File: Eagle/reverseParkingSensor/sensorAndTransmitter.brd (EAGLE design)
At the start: 42.2 x 52.1 mm, 31 parts, among them IC1 LM393N, IC3 MEGA8-P, Q1 BC558B, T1 BPX81, X1 YH-55-10

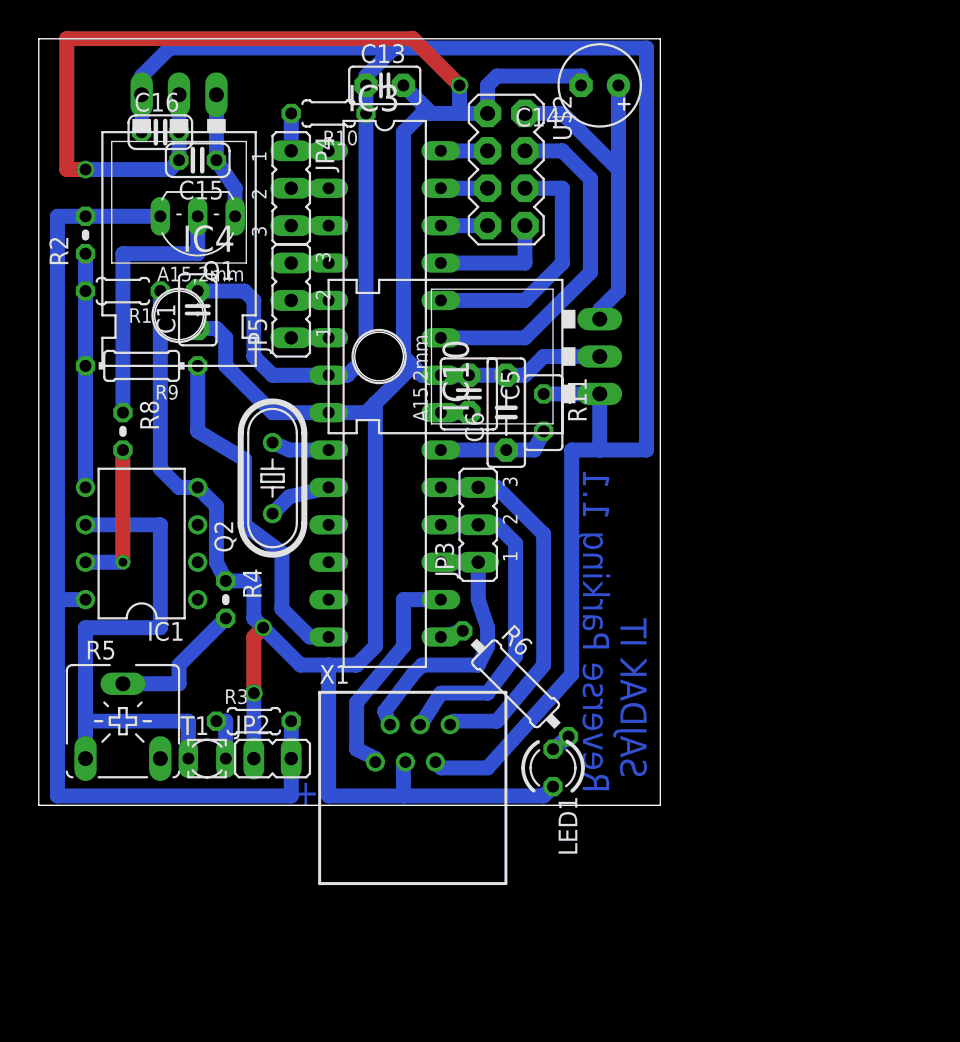
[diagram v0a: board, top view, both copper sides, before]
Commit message: final pcb
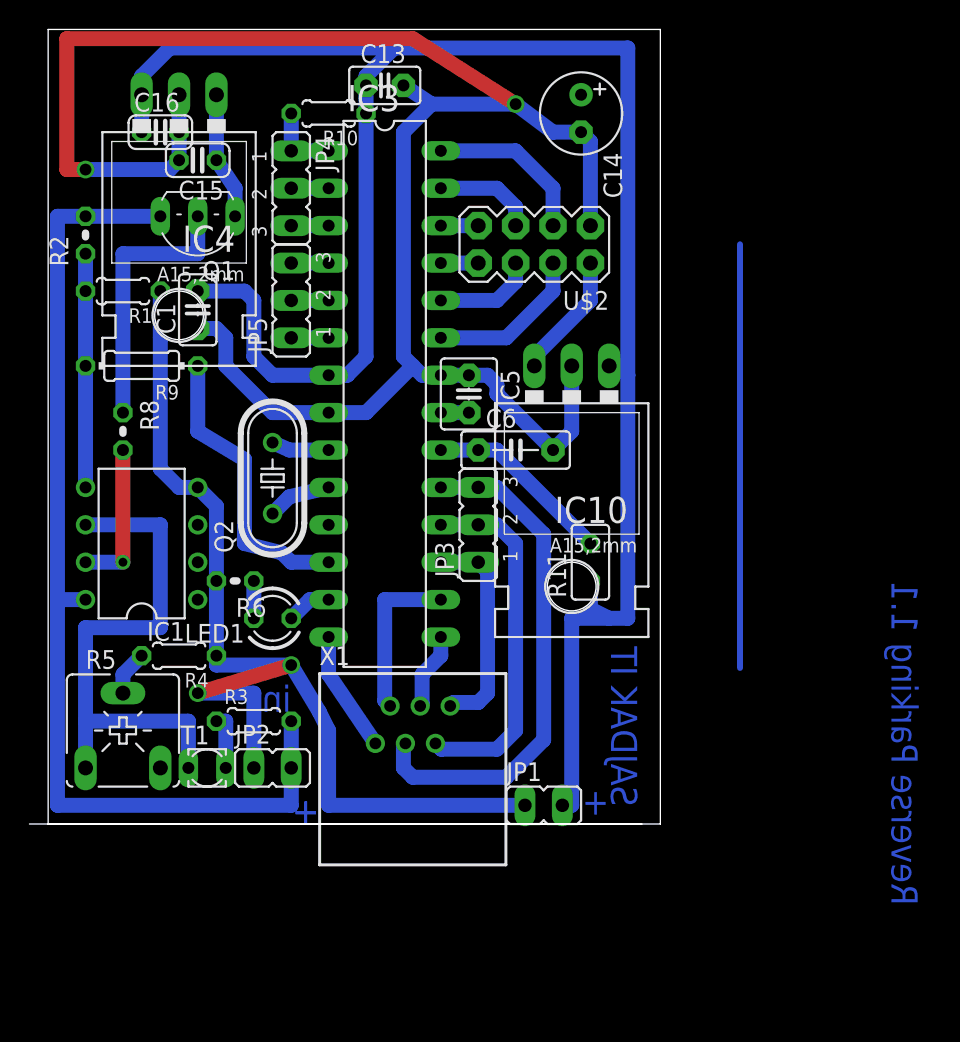
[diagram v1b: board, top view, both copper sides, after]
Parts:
- added JP1: (no value), jumper:JP1
- R4: device resistor:0204V -> resistor:0204/5
- R6: device resistor:0207/10 -> resistor:0204V
- moved LED1 21.6 mm to (41.9, 39.4), turned to 180 degrees
- moved R6 20.3 mm to (39.4, 41.9), turned to 180 degrees
- moved R11 10.6 mm to (63.5, 43.2), turned to 90 degrees
- moved U$2 5.43 mm to (59.7, 64.8), turned to 180 degrees
- moved R4 4.96 mm to (35.6, 36.8), turned to 180 degrees
- moved IC10 4.84 mm to (62.2, 52.7), turned to 180 degrees
- moved C6 2.62 mm to (58.4, 50.8), turned to 0 degrees
- moved C14 2.29 mm to (62.9, 73.7), turned to 270 degrees
- moved X1 1.27 mm to (51.4, 28.6)
- moved JP2 0.63 mm to (41.9, 29.2)
- moved R5 0.63 mm to (31.8, 31.8)
- moved T1 0.63 mm to (37.5, 29.2)
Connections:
- new net N$8: IC3.15, X1.4
- new net N$9: IC3.16, X1.2
- net +5V: now also JP1.2; no longer X1.5
- net GND: now also JP1.1, R6.2; no longer LED1.K, X1.3
- net N$5: now also IC3.14; no longer IC3.16
- net N$6: now also LED1.K; no longer IC3.15
- net N$7: now also IC3.13; no longer R6.2
- net PB3: now also X1.6; no longer X1.2
- net PB4: now also X1.5; no longer X1.4
- net PB5: now also X1.3; no longer X1.6
- net UPHOLD: now also IC3.12; no longer IC3.14
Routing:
- net N$11: track 0.00 -> 28.8 mm
- net +3V3: track 24.3 -> 8.56 mm
- net NRF_CSN: track 23.6 -> 10.8 mm
- net N$9: track 0.00 -> 11.2 mm
- net NRF_MOSI: track 16.9 -> 6.88 mm
- net PB5: track 25.4 -> 34.8 mm
- net NRF_CE: track 3.17 -> 11.2 mm
- net +5V: track 144.7 -> 136.7 mm
- net N$5: track 15.5 -> 8.20 mm
- net N$4: track 9.57 -> 3.07 mm
- net GND: track 210.8 -> 204.7 mm
- net NRF_IRQ: track 8.26 -> 2.54 mm
- net N$8: track 0.00 -> 5.27 mm
- net N$17: track 7.77 -> 12.8 mm
- net PB3: track 19.2 -> 14.6 mm
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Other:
- board size 42.2 x 52.1 mm -> 42.9 x 54 mm
- board text added: "in"
- board text removed: "C1"
- board text removed: "C2"
- board text removed: "C3"
- board text removed: "C4"
- board text removed: "C5"
- board text removed: "C6"
- board text removed: "C7"
- board text removed: "C8"
- board text removed: "IC1"
- board text removed: "IC2"
- board text removed: "IC3"
- board text removed: "IC4"
- board text removed: "IC5"
- board text removed: "IC6"
- board text removed: "J1"
- board text removed: "J2"
- board text removed: "J3"
- board text removed: "J4"
- board text removed: "JP11"
- board text removed: "JP12"
- board text removed: "JP13"
- board text removed: "JP3"
- board text removed: "JP4"
- board text removed: "JP6"
- board text removed: "Q1"
- board text removed: "R1"
- board text removed: "R10"
- board text removed: "R11"
- board text removed: "R12"
- board text removed: "R13"
- board text removed: "R14"
- board text removed: "R15"
- board text removed: "R16"
- board text removed: "R17"
- board text removed: "R18"
- board text removed: "R19"
- board text removed: "R2"
- board text removed: "R3"
- board text removed: "R4"
- board text removed: "R5"
- board text removed: "R6"
- board text removed: "R7"
- board text removed: "R8"
- board text removed: "R9"
- board text removed: "U$1"
- board text removed: "U$3"
- board text removed: "X3"
